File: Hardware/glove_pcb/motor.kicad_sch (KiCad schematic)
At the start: 5 parts, among them M1 Motor_DC, U2 DRV8848, U3 DRV8848, U4 DRV8848

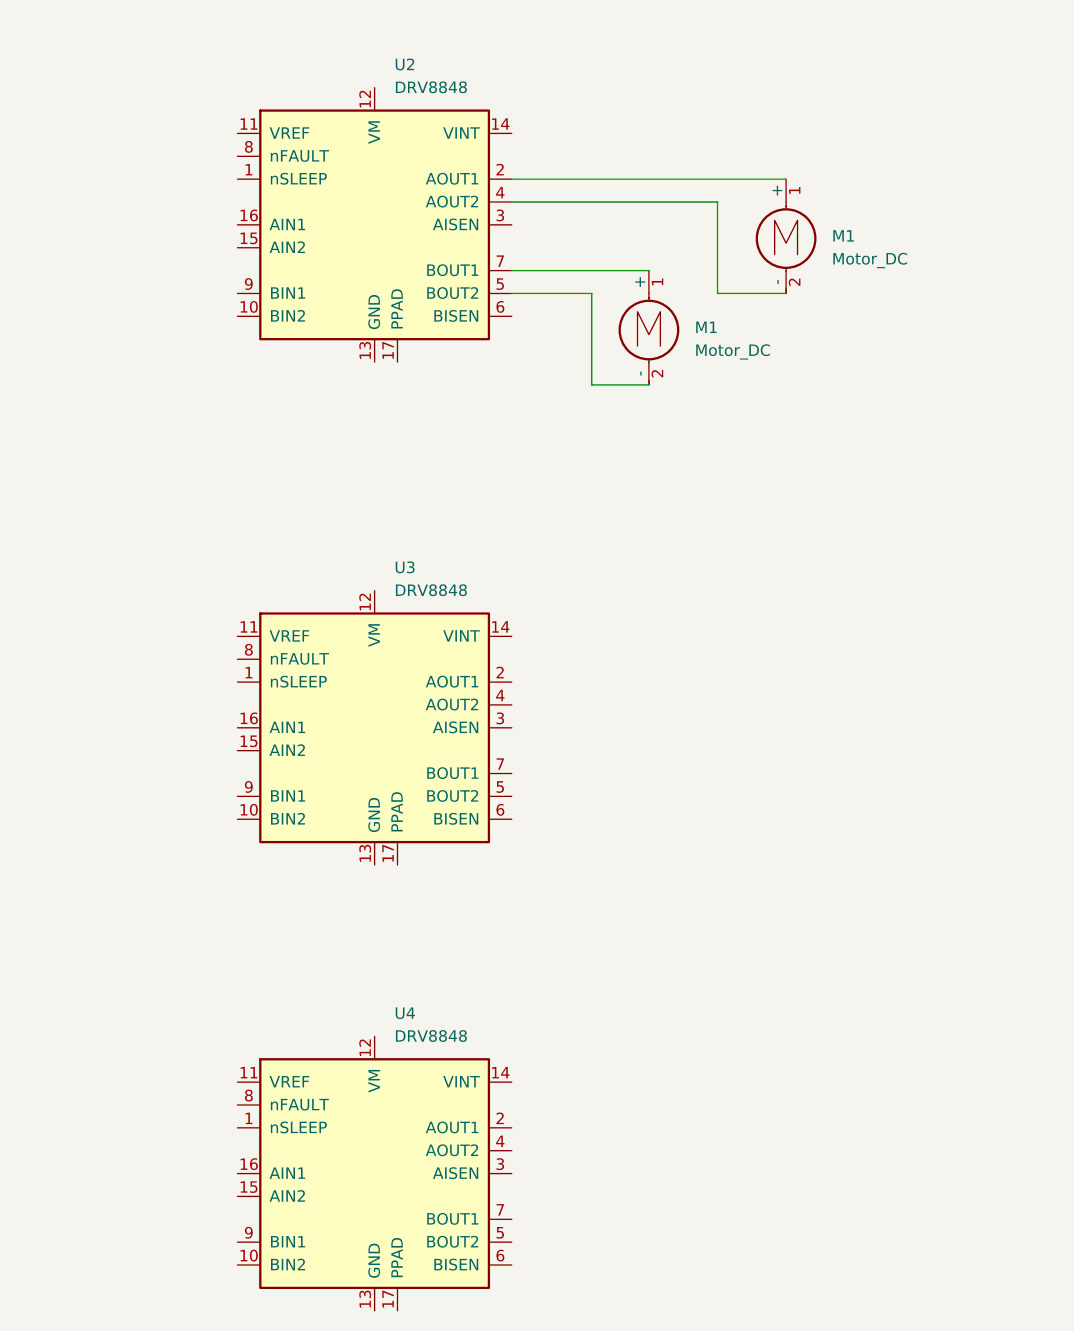
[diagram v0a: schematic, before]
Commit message: More work on motor driver connection
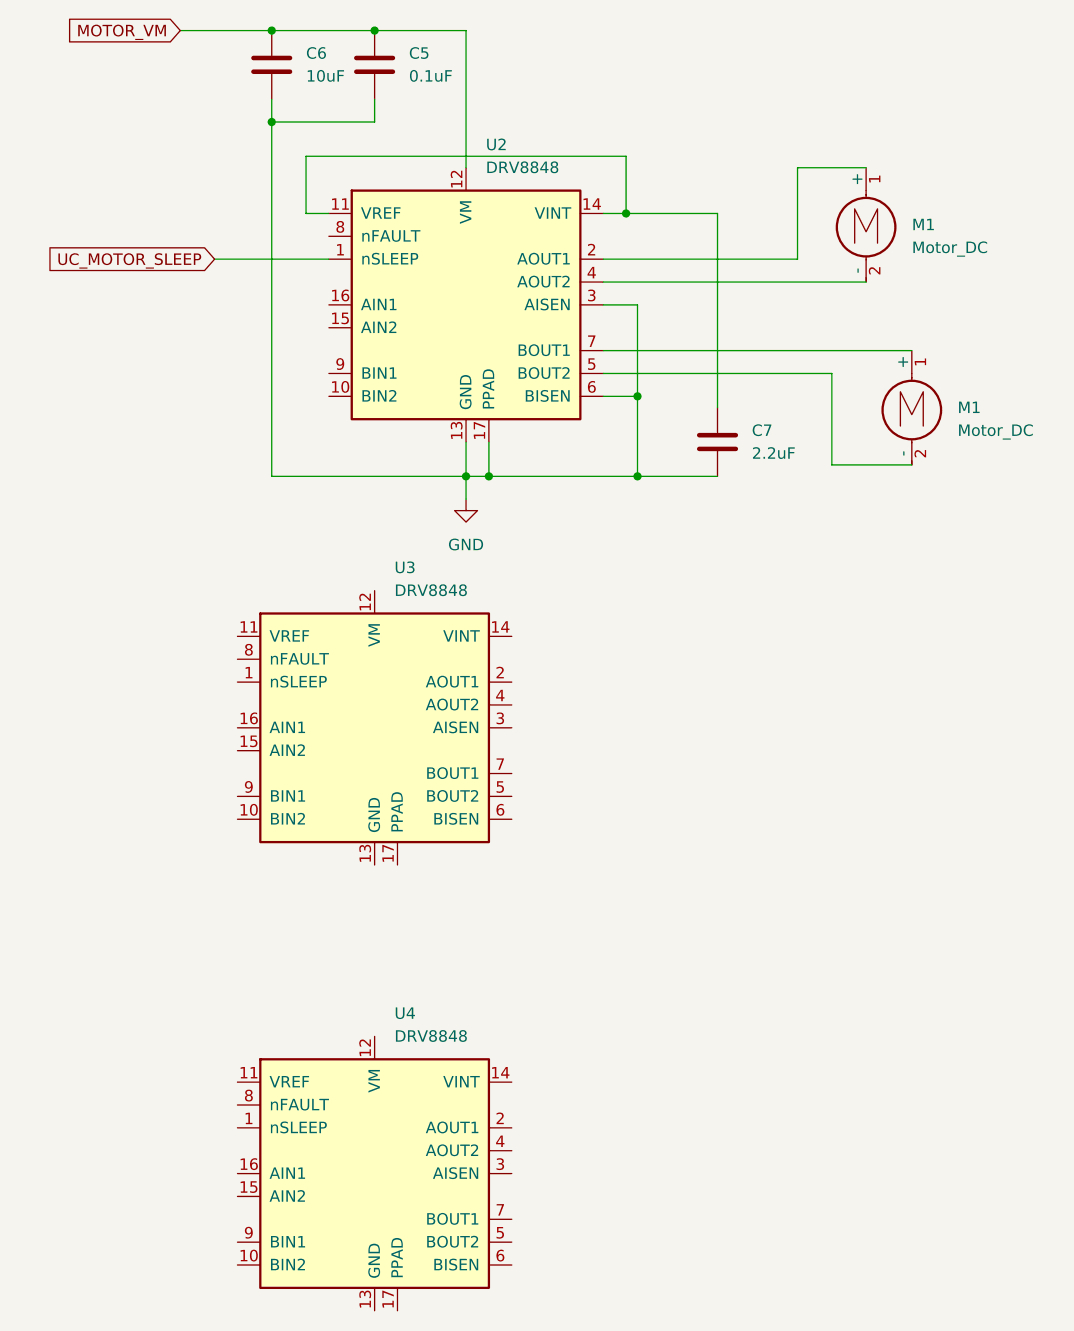
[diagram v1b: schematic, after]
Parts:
- added C5: 0.1uF, symbol Device:C
- added C6: 10uF, symbol Device:C
- added C7: 2.2uF, symbol Device:C
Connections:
- net UC_MOTOR_SLEEP: now reaches U2.1 (nSLEEP)
- net at U2.11 (VREF): now also U2.14 (VINT), C7.2
- net MOTOR_VM: now reaches U2.12 (VM)
- net MOTOR_VM: now also C5.1, C6.1
- net GND: now reaches U2.13 (GND)
- net GND: now also U2.17 (PPAD), U2.3 (AISEN), U2.6 (BISEN), C5.2, C6.2, C7.1
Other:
- moved on the sheet: M1, U2
